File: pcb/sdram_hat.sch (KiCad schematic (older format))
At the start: 34 parts, among them J1 CONN_02X20, J2 CONN_02X20, J3 CONN_02X20, J4 CONN_02X20, J5 AUDIO_OUT_JACK

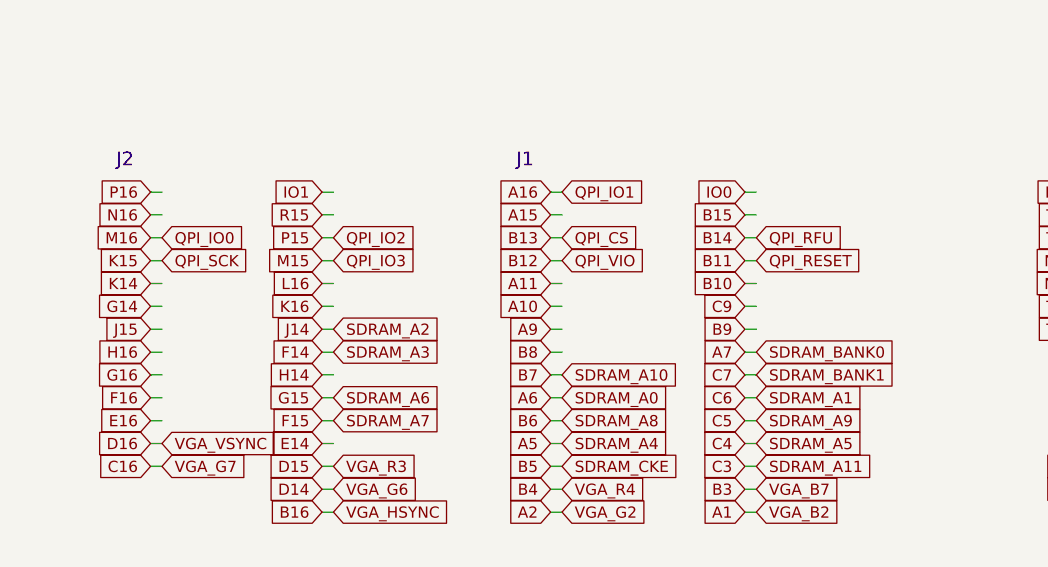
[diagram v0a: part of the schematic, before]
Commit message: Very misalign. Wow. Much fix.
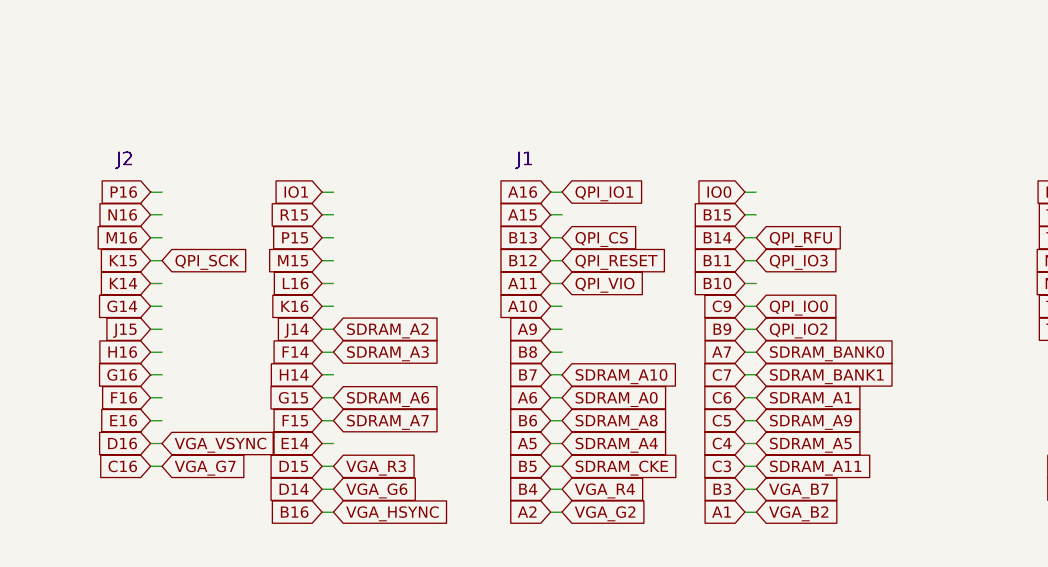
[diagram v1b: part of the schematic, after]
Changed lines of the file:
@@
 Text GLabel 11650 4400 2    49   Input ~ 0
 SDRAM_D0
-Text GLabel 9200 4000 2    49   Input ~ 0
+Text GLabel 8350 4000 2    49   Input ~ 0
 QPI_RESET
 Text GLabel 9200 3900 2    49   Input ~ 0
@@
 Text GLabel 6600 4000 2    49   Input ~ 0
 QPI_SCK
-Text GLabel 8350 4000 2    49   Input ~ 0
+Text GLabel 8350 4100 2    49   Input ~ 0
 QPI_VIO
 Text GLabel 8350 3900 2    49   Input ~ 0
 QPI_CS
-Text GLabel 6600 3900 2    49   Input ~ 0
+Text GLabel 9200 4200 2    49   Input ~ 0
 QPI_IO0
 Text GLabel 8350 3700 2    49   Input ~ 0
 QPI_IO1
-Text GLabel 7350 3900 2    49   Input ~ 0
+Text GLabel 9200 4300 2    49   Input ~ 0
 QPI_IO2
-Text GLabel 7350 4000 2    49   Input ~ 0
+Text GLabel 9200 4000 2    49   Input ~ 0
 QPI_IO3
 Text GLabel 11650 3900 2    49   Input ~ 0
